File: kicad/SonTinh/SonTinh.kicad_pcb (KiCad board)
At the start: 2 copper layers, 129 x 39 mm, 7 parts, among them J1 Screw_Terminal_01x02, J11 Conn_01x03_Socket, J2 Screw_Terminal_01x02, J3 Screw_Terminal_01x02, U1 BME680

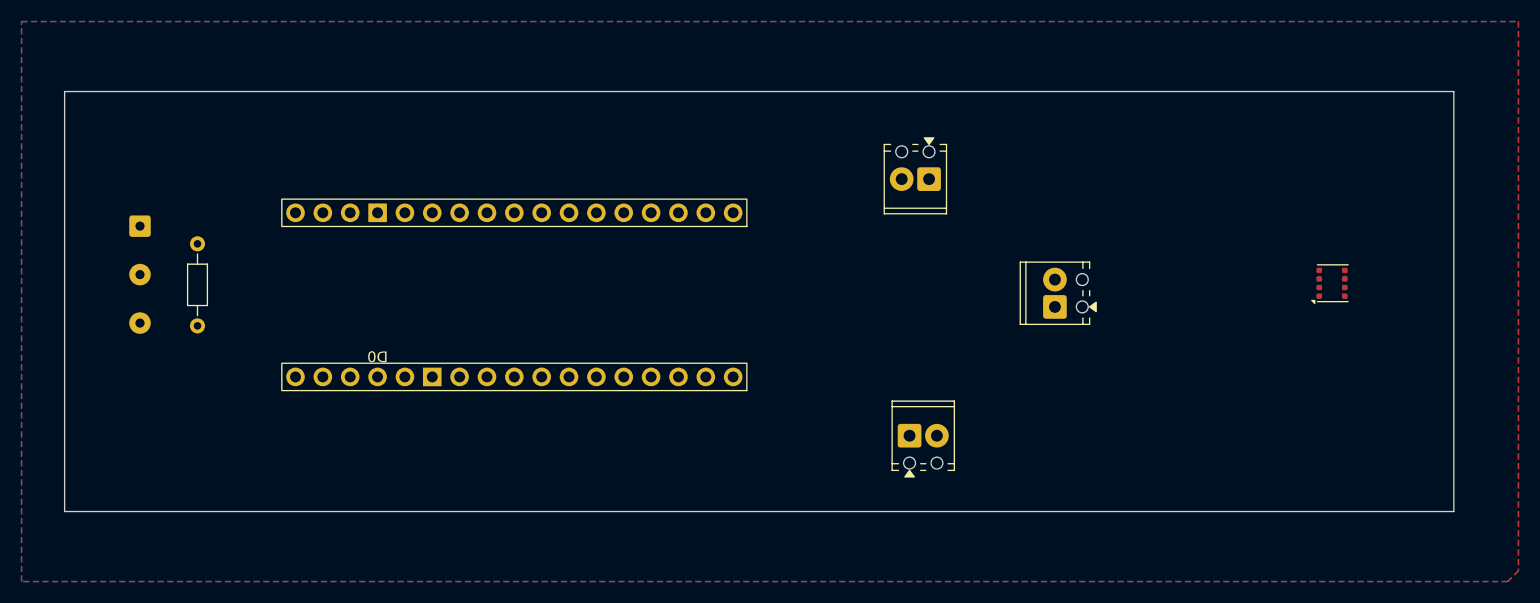
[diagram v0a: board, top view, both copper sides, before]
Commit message: Fins, Femmes and Gems
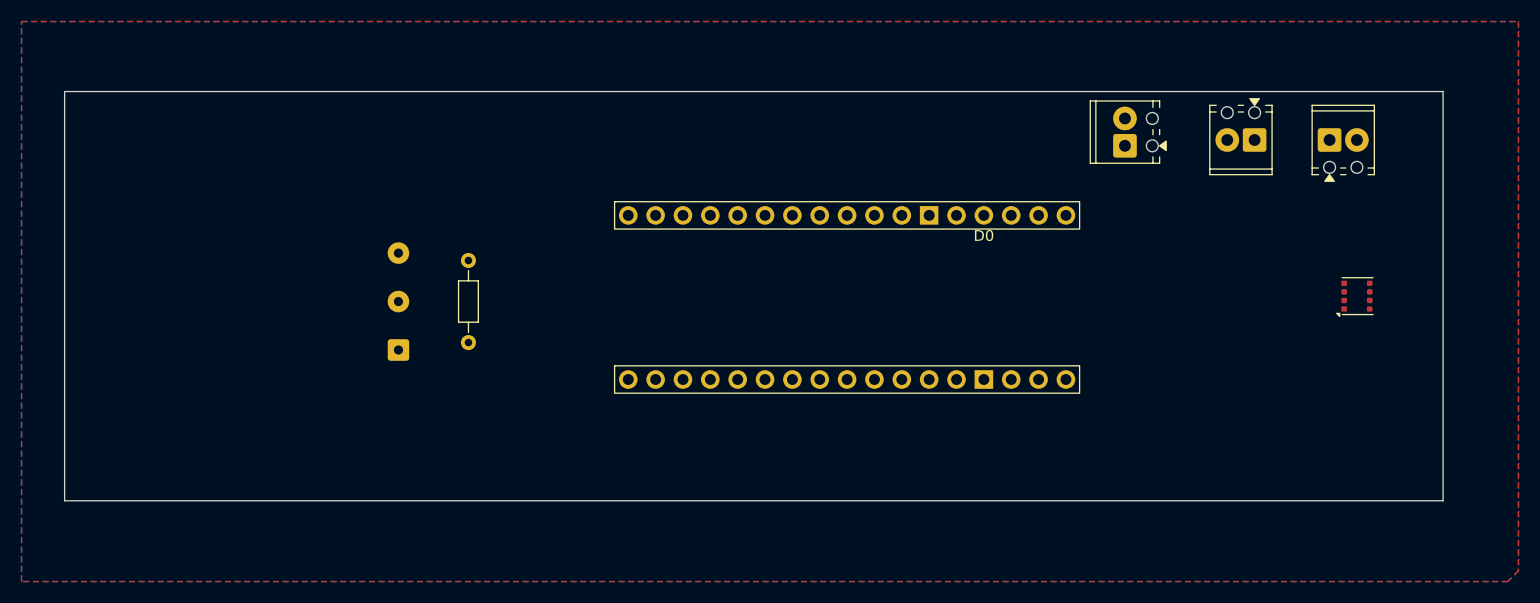
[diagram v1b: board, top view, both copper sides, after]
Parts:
- moved J1 47.7 mm to (158.3, 46.0)
- moved J2 30.4 mm to (151.3, 46.0)
- moved J11 26.6 mm to (71.8, 65.5), turned to 90 degrees
- moved R13 25.9 mm to (78.3, 57.2), turned to -90 degrees
- moved A1 25.3 mm to (89.3, 69.6), turned to 0 degrees
- moved J3 16.3 mm to (139.3, 46.5)
- moved U1 2.61 mm to (160.8, 60.5)
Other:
- board size 129 x 39 mm -> 128 x 38 mm
